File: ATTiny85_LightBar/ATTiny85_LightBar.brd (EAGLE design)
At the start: 25.4 x 47.9 mm, 8 parts, among them U1 ATTINY85-20P, X1 JST-XH-02-PIN-ROUND-PAD, X2 JST-XH-02-PIN-ROUND-PAD, X3 JST-XH-03-PIN-ROUND-PAD

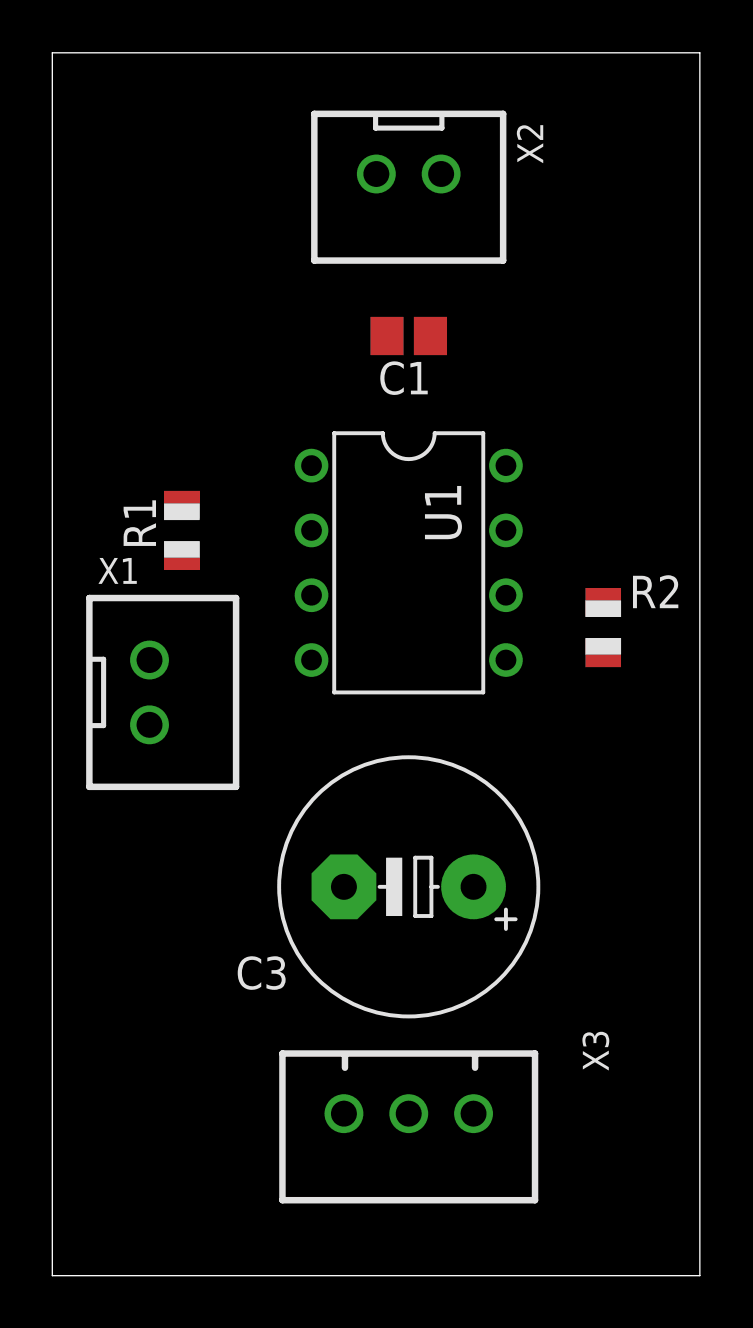
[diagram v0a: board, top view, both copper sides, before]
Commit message: updating corrected files for PCB
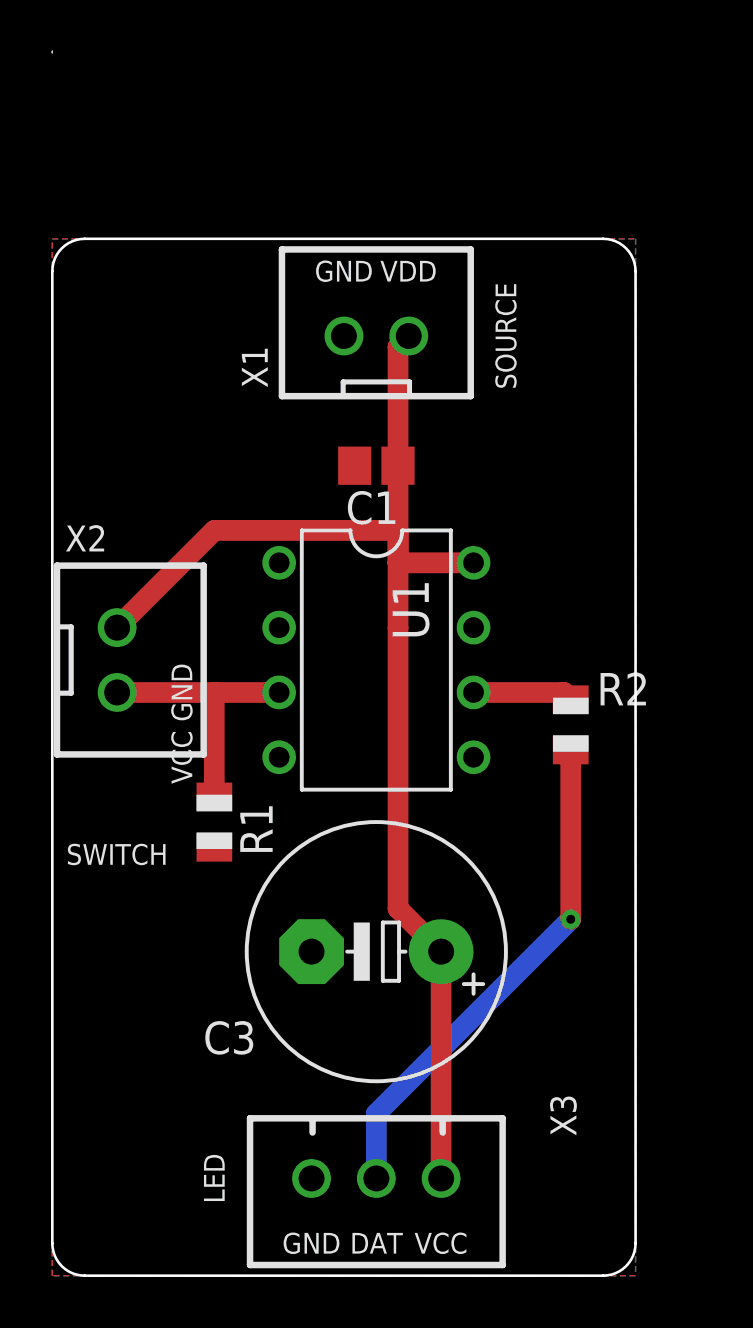
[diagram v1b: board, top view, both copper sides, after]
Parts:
- moved X2 22.2 mm to (2.54, 24.1), turned to 270 degrees
- moved X1 16.6 mm to (12.7, 36.8), turned to 0 degrees
- moved R1 11.5 mm to (6.35, 17.8), turned to 270 degrees
- moved C1 5.24 mm to (12.7, 31.8)
- moved U1 4.02 mm to (12.7, 24.1)
- moved R2 4.02 mm to (20.3, 21.6)
- moved C3 2.84 mm to (12.7, 12.7)
- moved X3 2.84 mm to (12.7, 3.81)
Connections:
- removed net N$1: C1.1, U1.8, X1.2
- net N$2: now also X2.2; no longer X2.1
- net VCC: now also C1.1, U1.8, X1.2, X2.1; no longer X2.2
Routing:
- net VCC: track 0.00 -> 50.7 mm
- net N$5: track 0.00 -> 19.9 mm, vias 0 -> 1
- net N$2: track 0.00 -> 10.4 mm
- net N$4: track 0.00 -> 3.92 mm
- added copper zone on layer 1, net GND
- added copper zone on layer 16, net GND
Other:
- board size 25.4 x 47.9 mm -> 22.9 x 48 mm
- board text added: "DAT"
- board text added: "GND"
- board text added: "LED"
- board text added: "SOURCE"
- board text added: "SWITCH"
- board text added: "VCC"
- board text added: "VDD"
